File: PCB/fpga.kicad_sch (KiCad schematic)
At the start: 76 parts, among them IC1 S25FL256LAGMFI003, J1 0878311420, J4 62684-402100ALF, U4 XC7A100T-FTG256, U5 IS62C1024AL-35QLI-TR, Y2 ECS-3953M-400-BN-TR

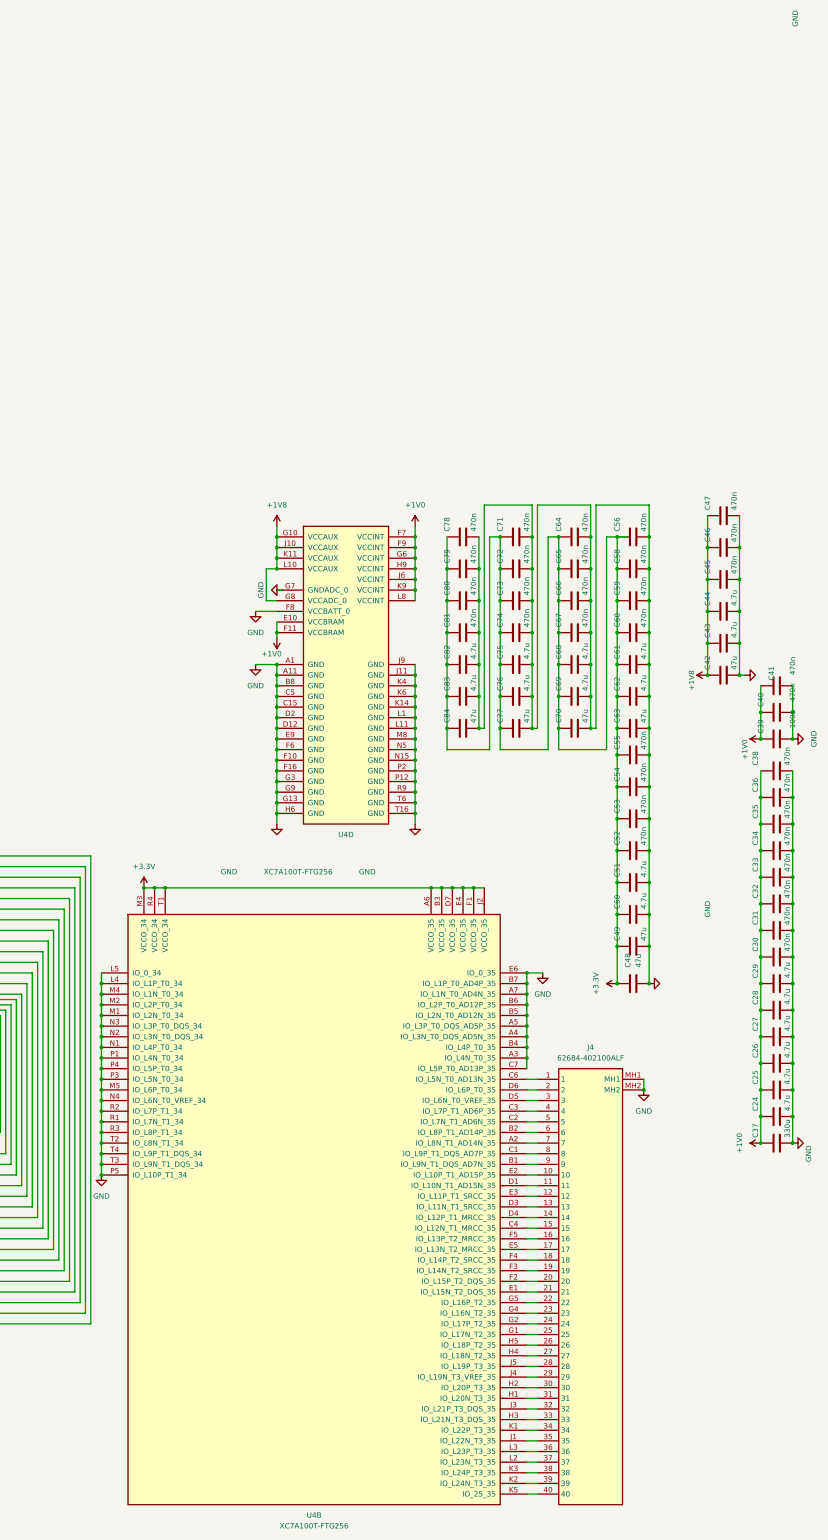
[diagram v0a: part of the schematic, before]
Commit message: Add
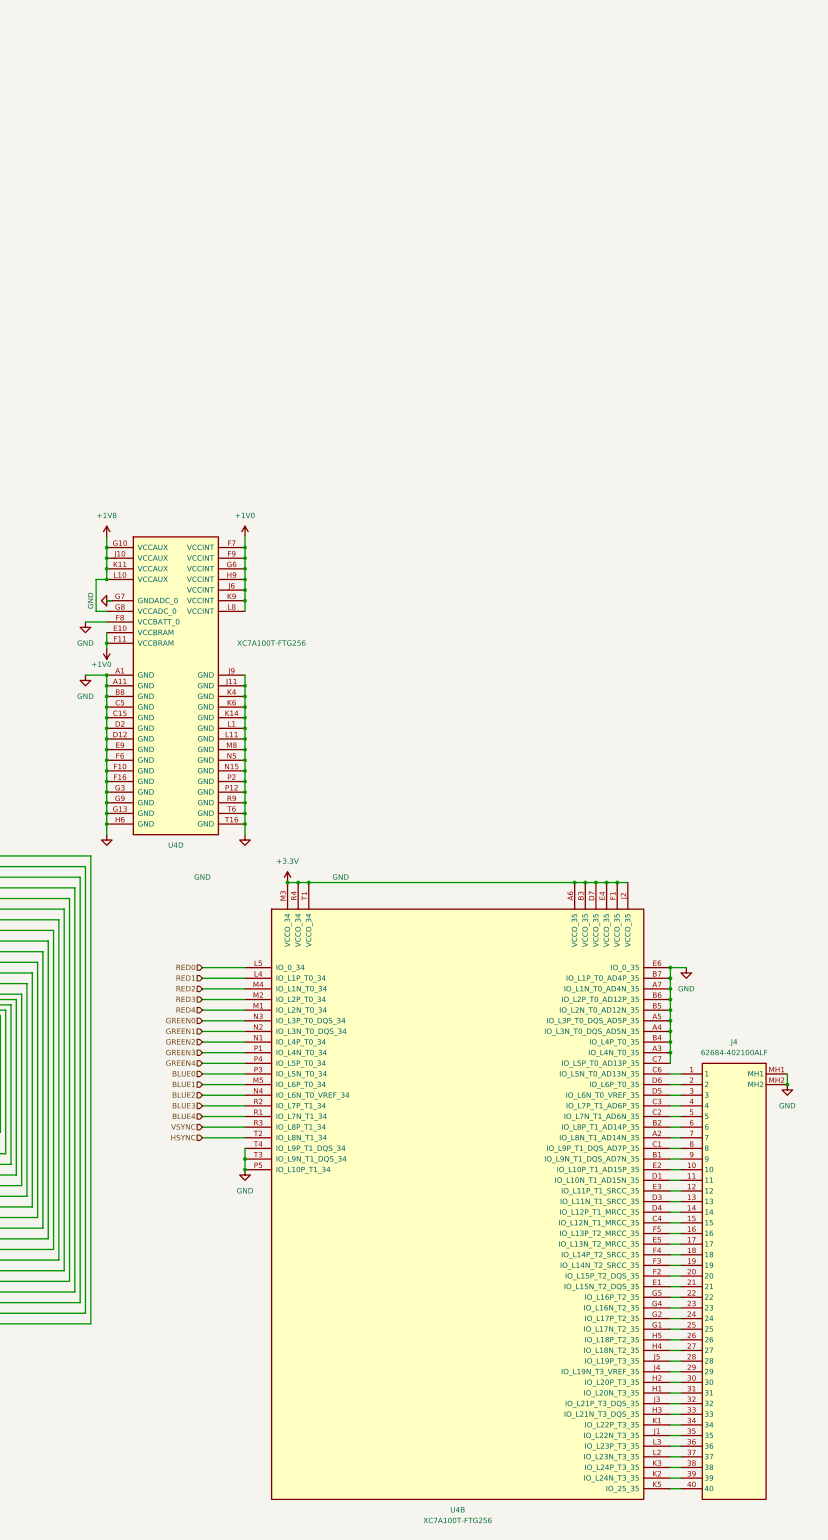
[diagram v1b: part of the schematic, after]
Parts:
- removed C24, C25, C26, C27, C28, C29, C43, C44, C50, C51, C61, C62, C68, C69, C75, C76, C82, C83: 4.7u, symbol Device:C
- removed C30, C31, C32, C33, C34, C35, C36, C38, C40, C41, C45, C46, C47, C52, C53, C54, C55, C56, C58, C59, C60, C64, C65, C66, C67, C71, C72, C73, C74, C78, C79, C80, C81: 470n, symbol Device:C
- removed C37: 330u, symbol Device:C
- removed C39: 100u, symbol Device:C
- removed C42, C48, C49, C63, C70, C77, C84: 47u, symbol Device:C
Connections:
- net GND: no longer U4.L4 (IO_L1P_T0_34), U4.L5 (IO_0_34), U4.M1 (IO_L2N_T0_34), U4.M2 (IO_L2P_T0_34), U4.M4 (IO_L1N_T0_34), U4.M5 (IO_L6P_T0_34), U4.N1 (IO_L4P_T0_34), U4.N2 (IO_L3N_T0_DQS_34), U4.N3 (IO_L3P_T0_DQS_34), U4.N4 (IO_L6N_T0_VREF_34), U4.P1 (IO_L4N_T0_34), U4.P3 (IO_L5N_T0_34), U4.P4 (IO_L5P_T0_34), U4.R1 (IO_L7N_T1_34), U4.R2 (IO_L7P_T1_34), U4.R3 (IO_L8P_T1_34), U4.T2 (IO_L8N_T1_34)
- new net BLUE0: U4.P3 (IO_L5N_T0_34)
- new net BLUE1: U4.M5 (IO_L6P_T0_34)
- new net BLUE2: U4.N4 (IO_L6N_T0_VREF_34)
- new net BLUE3: U4.R2 (IO_L7P_T1_34)
- new net BLUE4: U4.R1 (IO_L7N_T1_34)
- new net GREEN0: U4.N3 (IO_L3P_T0_DQS_34)
- new net GREEN1: U4.N2 (IO_L3N_T0_DQS_34)
- new net GREEN2: U4.N1 (IO_L4P_T0_34)
- new net GREEN3: U4.P1 (IO_L4N_T0_34)
- new net GREEN4: U4.P4 (IO_L5P_T0_34)
- new net HSYNC: U4.T2 (IO_L8N_T1_34)
- new net RED0: U4.L5 (IO_0_34)
- new net RED1: U4.L4 (IO_L1P_T0_34)
- new net RED2: U4.M4 (IO_L1N_T0_34)
- new net RED3: U4.M2 (IO_L2P_T0_34)
- new net RED4: U4.M1 (IO_L2N_T0_34)
- new net VSYNC: U4.R3 (IO_L8P_T1_34)
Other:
- moved on the sheet: J4, U4B, U4D
